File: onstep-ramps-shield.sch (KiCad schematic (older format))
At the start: 24 parts

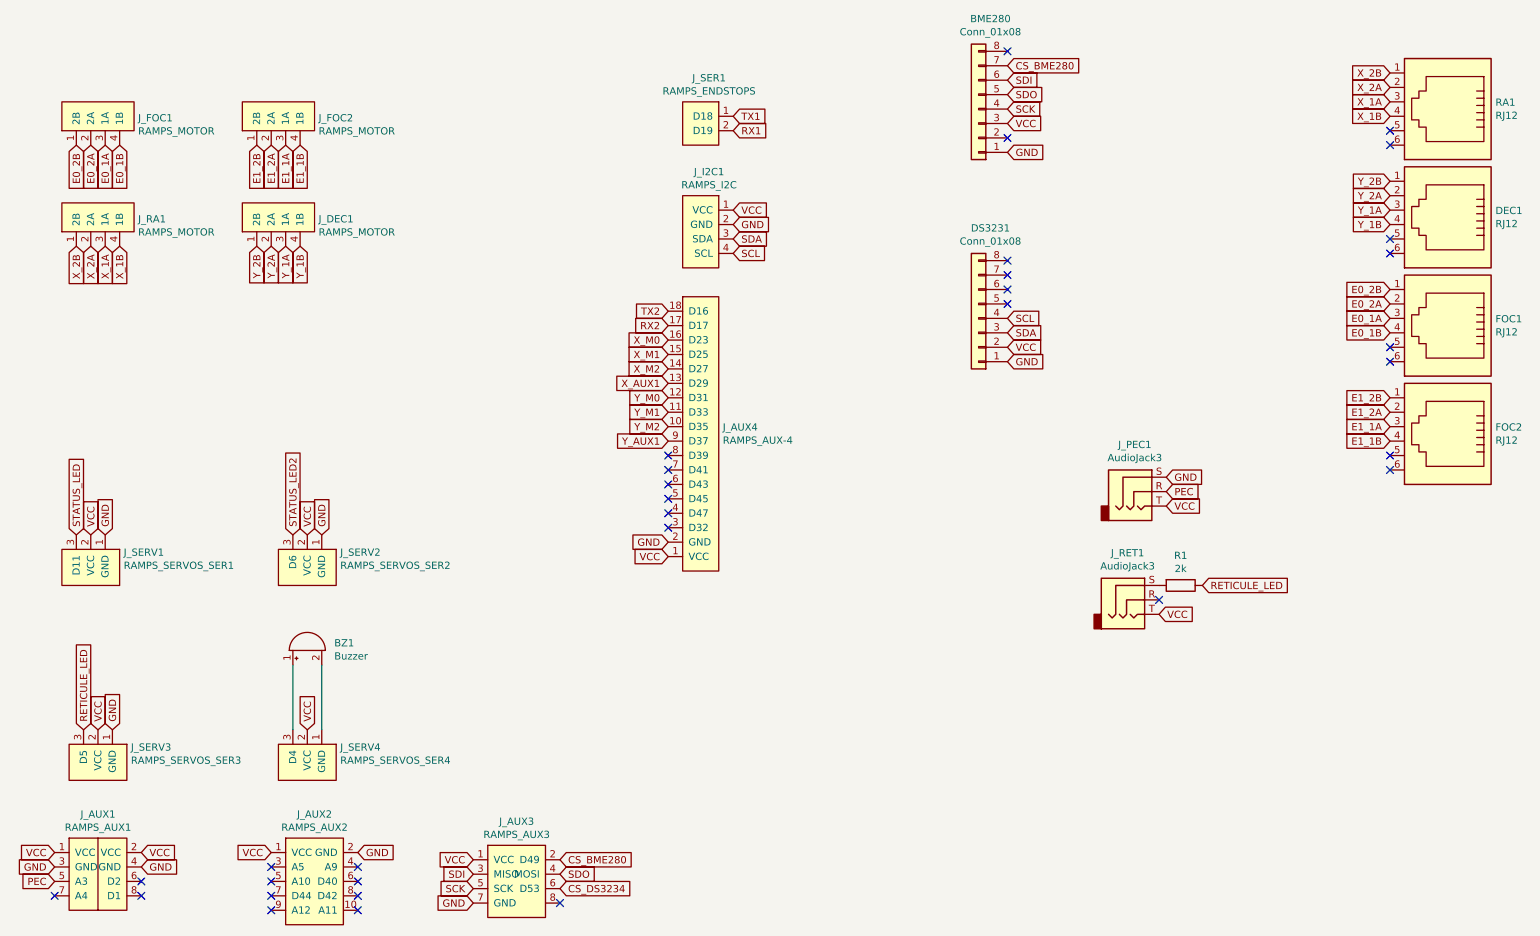
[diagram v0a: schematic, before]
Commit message: Routing
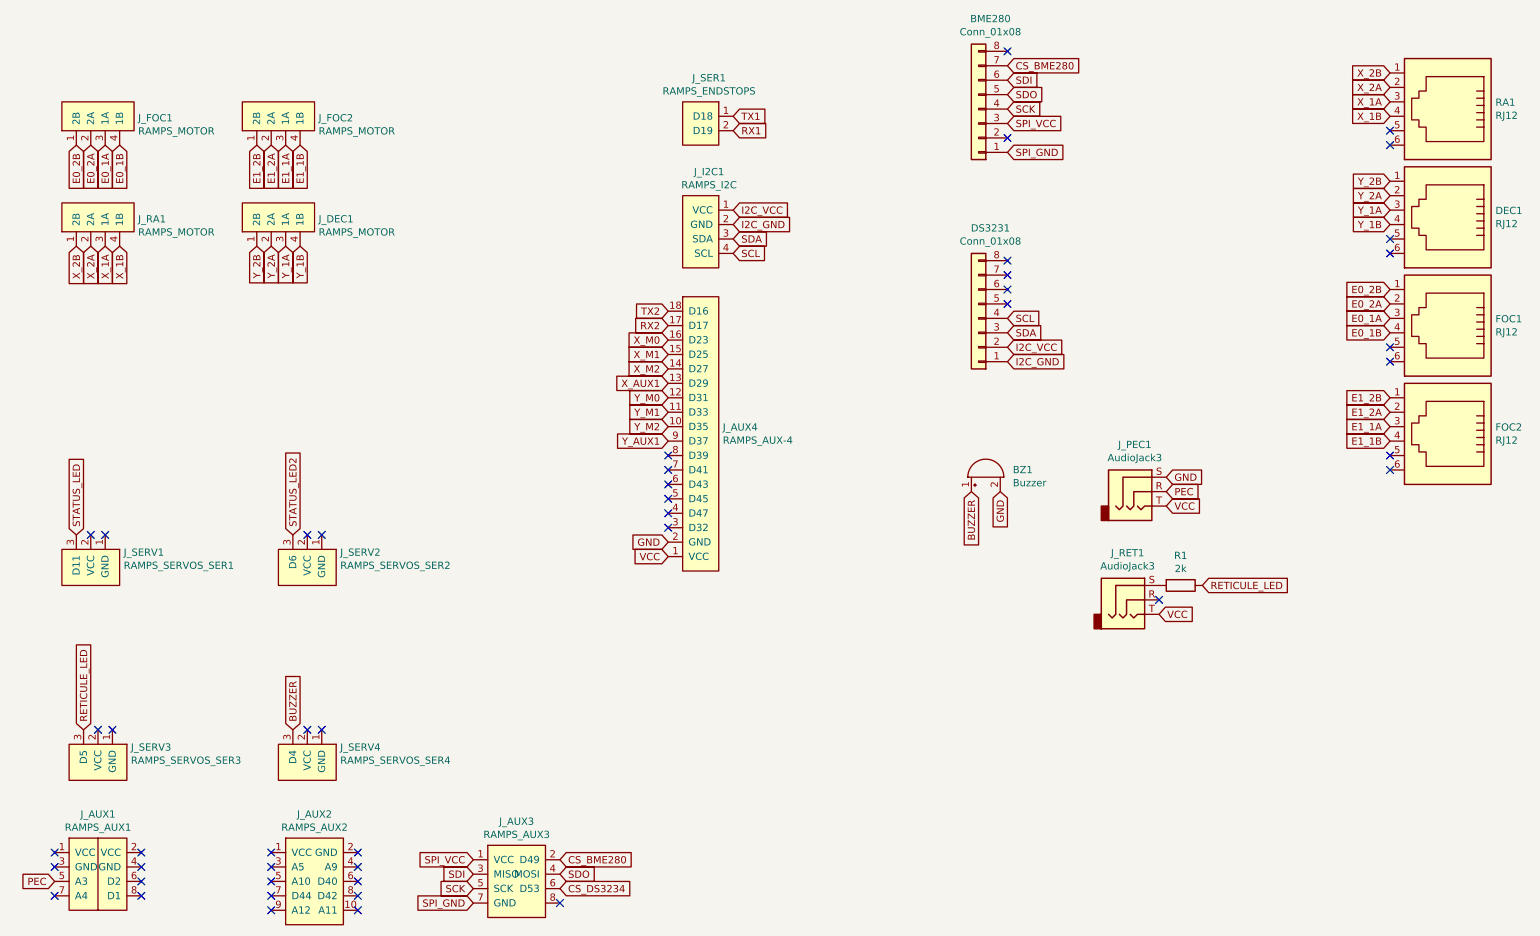
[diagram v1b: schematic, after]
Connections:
- net GND: now also BZ1.2 (+); no longer BME280.1 (Pin_1), DS3231.1 (Pin_1), J_AUX1.3 (GND), J_AUX1.4 (GND), J_AUX2.2 (GND), J_AUX3.7 (GND), J_I2C1.2 (GND), J_SERV1.1 (GND), J_SERV2.1 (GND), J_SERV3.1 (GND)
- net VCC: no longer BME280.3 (Pin_3), DS3231.2 (Pin_2), J_AUX1.1 (VCC), J_AUX1.2 (VCC), J_AUX2.1 (VCC), J_AUX3.1 (VCC), J_I2C1.1 (VCC), J_SERV1.2 (VCC), J_SERV2.2 (VCC), J_SERV3.2 (VCC), J_SERV4.2 (VCC)
- net at J_SERV4.1 (GND): no longer BZ1.2 (+)
- net BUZZER: now reaches BZ1.1 (-), J_SERV4.3 (D4)
- new net I2C_GND: DS3231.1 (Pin_1), J_I2C1.2 (GND)
- new net I2C_VCC: DS3231.2 (Pin_2), J_I2C1.1 (VCC)
- new net SPI_GND: BME280.1 (Pin_1), J_AUX3.7 (GND)
- new net SPI_VCC: BME280.3 (Pin_3), J_AUX3.1 (VCC)
- no-connect marks 33 -> 47
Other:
- moved on the sheet: BZ1
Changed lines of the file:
@@
 	0    -1   -1   0
 $EndComp
-Text GLabel 2350 6700 0    50   Input ~ 0
-VCC
-Text GLabel 3750 6750 0    50   Input ~ 0
-VCC
 Text GLabel 5100 4650 0    50   Input ~ 0
 VCC
 Text GLabel 5550 2250 2    50   Input ~ 0
-VCC
-Text GLabel 2950 6700 2    50   Input ~ 0
-GND
-Text GLabel 3750 7050 0    50   Input ~ 0
-GND
+I2C_VCC
 Text GLabel 5100 4550 0    50   Input ~ 0
 GND
 Text GLabel 5550 2350 2    50   Input ~ 0
-GND
+I2C_GND
 Text GLabel 1000 1800 3    50   Input ~ 0
 E0_2B
@@
 L Device:Buzzer BZ1
 U 1 1 5F550329
-P 2600 5300
-F 0 "BZ1" V 2651 5113 50  0000 R CNN
-F 1 "Buzzer" V 2560 5113 50  0000 R CNN
-F 2 "Buzzer_Beeper:Buzzer_12x9.5RM7.6" V 2575 5400 50  0001 C CNN
-F 3 "~" V 2575 5400 50  0001 C CNN
-	1    2600 5300
-	0    -1   -1   0
-$EndComp
-Wire Wire Line
-	2500 5850 2500 5400
-Wire Wire Line
-	2700 5400 2700 5850
+P 7300 4100
+F 0 "BZ1" V 7351 3913 50  0000 R CNN
+F 1 "Buzzer" V 7260 3913 50  0000 R CNN
+F 2 "Buzzer_Beeper:Buzzer_12x9.5RM7.6" V 7275 4200 50  0001 C CNN
+F 3 "~" V 7275 4200 50  0001 C CNN
+	1    7300 4100
+	0    -1   -1   0
+$EndComp
 Text GLabel 4350 6950 2    50   Input ~ 0
 CS_DS3234
@@
 Text GLabel 7450 1250 2    50   Input ~ 0
 CS_BME280
-Text GLabel 7450 1850 2    50   Input ~ 0
-GND
-Text GLabel 7450 1650 2    50   Input ~ 0
-VCC
-Text GLabel 7450 3200 2    50   Input ~ 0
-VCC
 Text GLabel 7450 3300 2    50   Input ~ 0
-GND
+I2C_GND
 Text GLabel 4350 6750 2    50   Input ~ 0
 CS_BME280
@@
 	0    -1   -1   0
 $EndComp
-Text GLabel 1450 6800 2    50   Input ~ 0
-GND
-Text GLabel 1450 6700 2    50   Input ~ 0
-VCC
-Text GLabel 850  6800 0    50   Input ~ 0
-GND
-Text GLabel 850  6700 0    50   Input ~ 0
-VCC
-Text GLabel 2700 4500 1    50   Input ~ 0
-GND
-Text GLabel 2600 4500 1    50   Input ~ 0
-VCC
-Text GLabel 2600 5850 1    50   Input ~ 0
-VCC
-Text GLabel 1250 5850 1    50   Input ~ 0
-GND
-Text GLabel 1150 5850 1    50   Input ~ 0
-VCC
-Text GLabel 1200 4500 1    50   Input ~ 0
-GND
-Text GLabel 1100 4500 1    50   Input ~ 0
-VCC
 $Comp
 L Connector_Generic:Conn_01x08 BME280
@@
 NoConn ~ 7450 2700
 NoConn ~ 7450 2600
+Text GLabel 7450 3200 2    50   Input ~ 0
+I2C_VCC
+Text GLabel 3750 6750 0    50   Input ~ 0
+SPI_VCC
+Text GLabel 3750 7050 0    50   Input ~ 0
+SPI_GND
+Text GLabel 7450 1650 2    50   Input ~ 0
+SPI_VCC
+Text GLabel 7450 1850 2    50   Input ~ 0
+SPI_GND
+NoConn ~ 2600 4500
+NoConn ~ 2700 4500
+NoConn ~ 1100 4500
+NoConn ~ 1200 4500
+NoConn ~ 1150 5850
+NoConn ~ 1250 5850
+NoConn ~ 2600 5850
+NoConn ~ 2700 5850
+Text GLabel 2500 5850 1    50   Input ~ 0
+BUZZER
+Text GLabel 7200 4200 3    50   Input ~ 0
+BUZZER
+Text GLabel 7400 4200 3    50   Input ~ 0
+GND
+NoConn ~ 2350 6700
+NoConn ~ 2950 6700
+NoConn ~ 850  6700
+NoConn ~ 850  6800
+NoConn ~ 1450 6800
+NoConn ~ 1450 6700
 $EndSCHEMATC
